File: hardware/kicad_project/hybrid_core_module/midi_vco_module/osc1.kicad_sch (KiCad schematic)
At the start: 57 parts, among them Q12 SSM2212, Q14 BF545A, Q15 2N7002, Q16 2N7002, U11 TL074, U12 LM311DR, U13 TL072

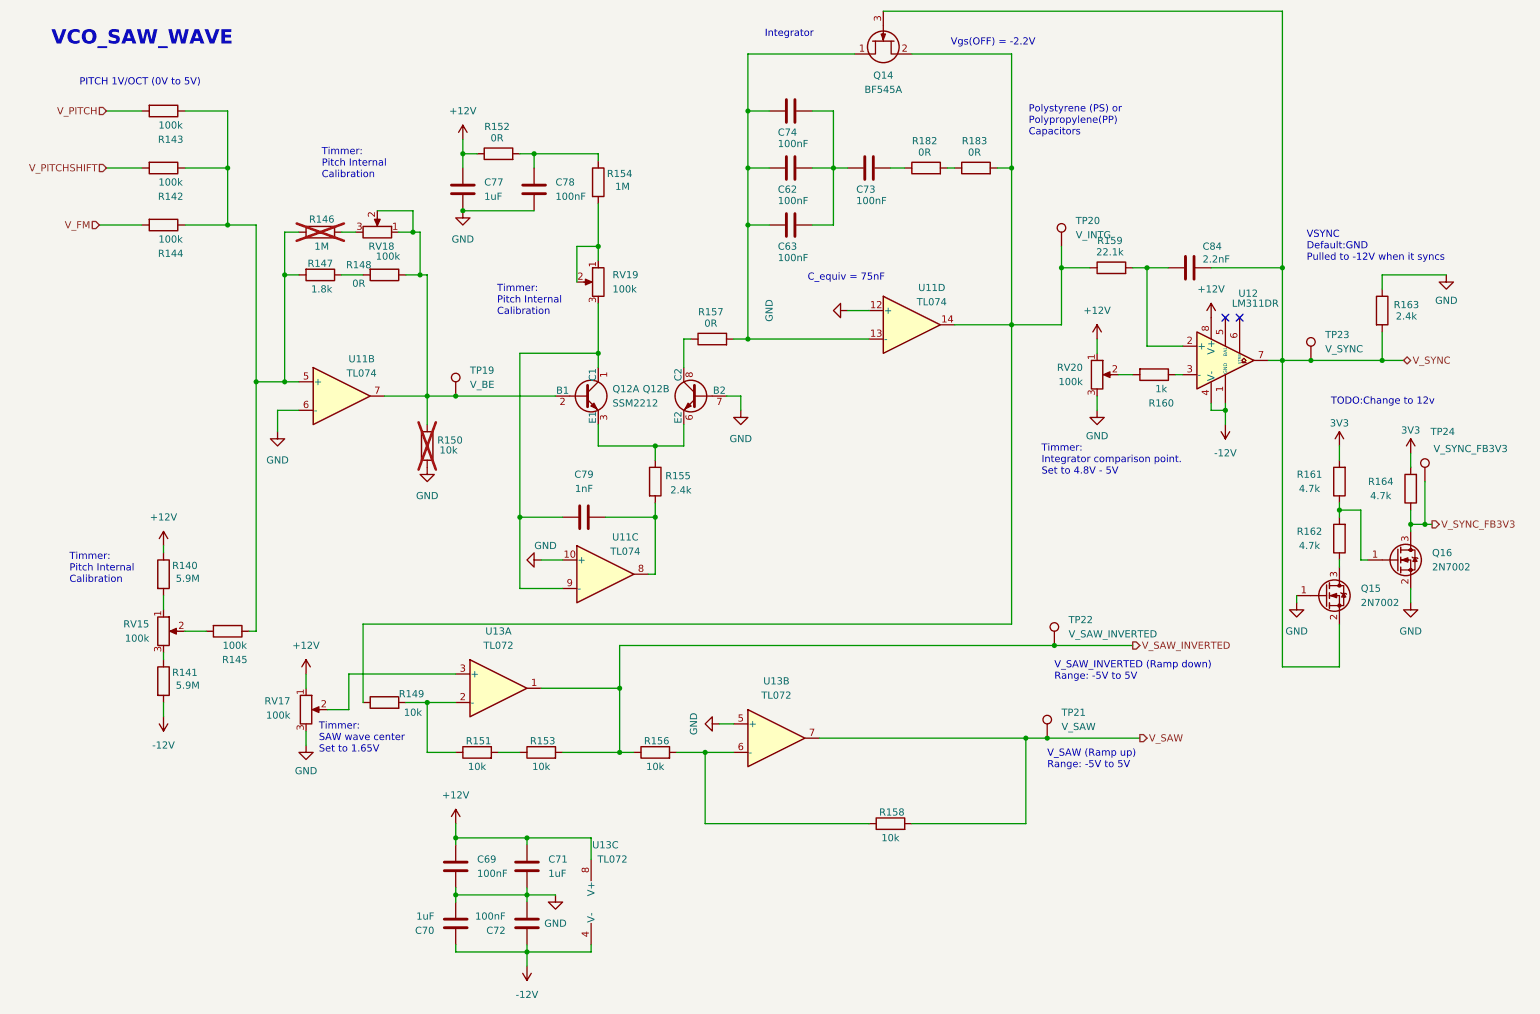
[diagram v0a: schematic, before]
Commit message: - placement done - routing 60%
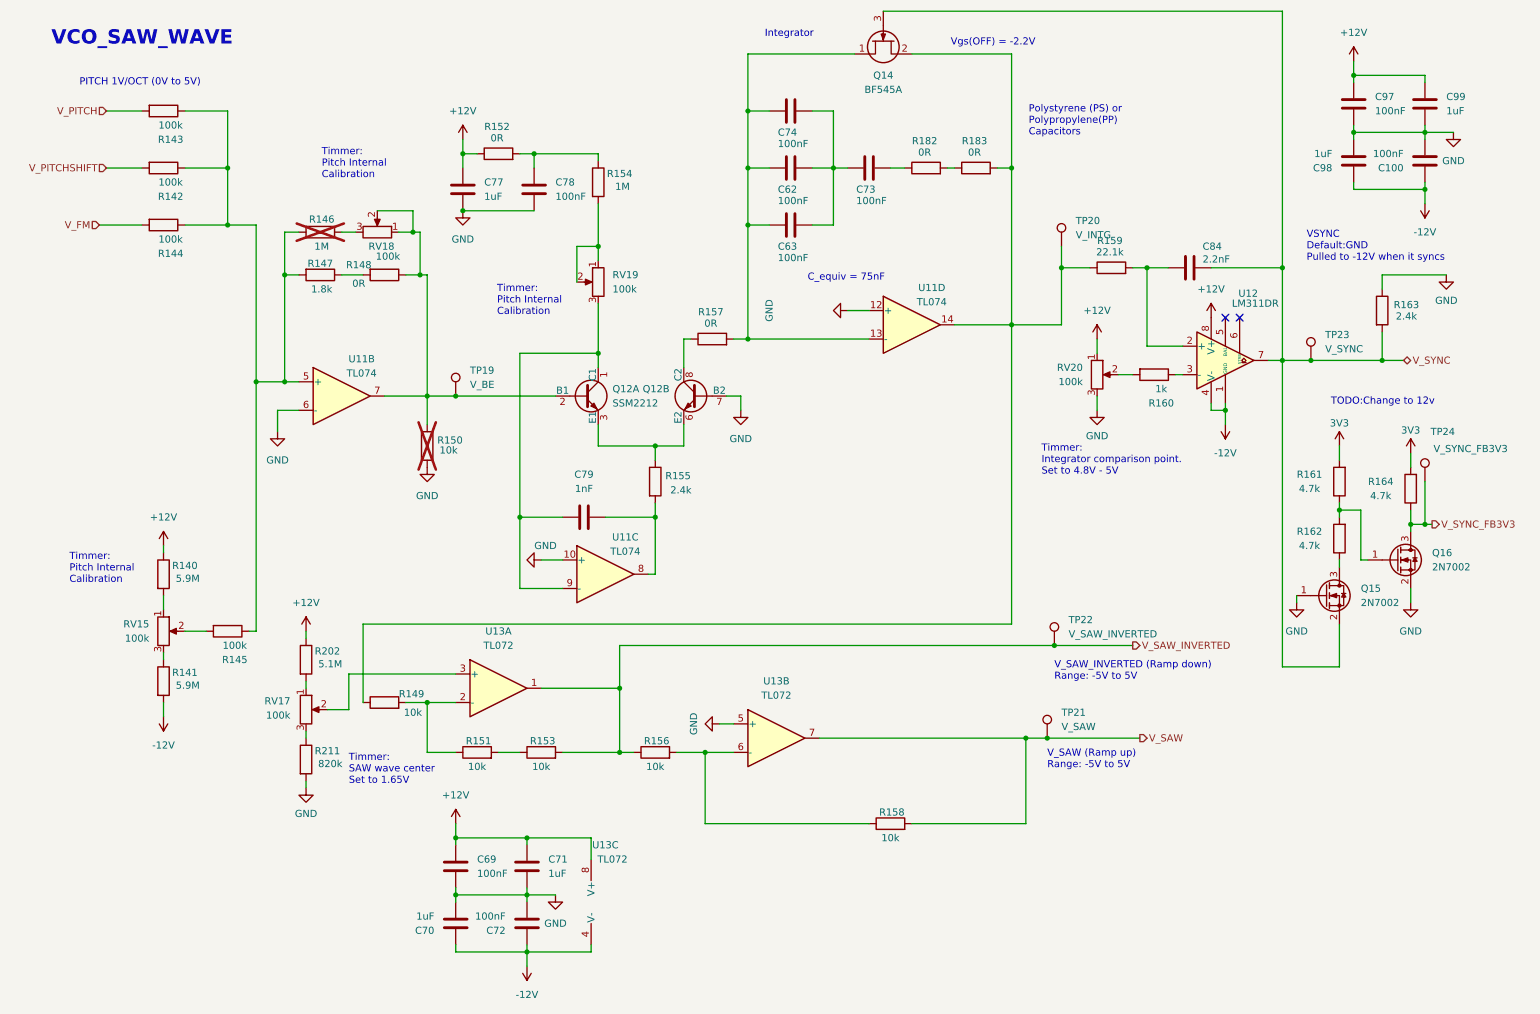
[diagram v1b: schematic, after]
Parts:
- added C100, C97: 100nF, Capacitor_SMD:C_0402_1005Metric, symbol Device:C
- added C98, C99: 1uF, Capacitor_SMD:C_0805_2012Metric, symbol Device:C
- added R202: 5.1M, Resistor_SMD:R_0402_1005Metric, symbol Device:R
- added R211: 820k, Resistor_SMD:R_0402_1005Metric, symbol Device:R
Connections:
- net +12V: now also C97.1, C99.1, R202.1; no longer RV17.1
- net -12V: now also C100.1, C98.1
- net GND: now also C100.2, C97.2, C98.2, C99.2, R211.2; no longer RV17.3
- new net: R202.2, RV17.1
- new net: R211.1, RV17.3

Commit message: routing continued.
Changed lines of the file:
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@@
 		(lib_id "power:+15V")
 		(at 41.91 111.76 0)
+		(mirror y)
 		(unit 1)
 		(exclude_from_sim no)
@@
 		(on_board yes)
 		(dnp no)
-		(fields_autoplaced yes)
 		(property "Reference" "#PWR0279"
 			(at 41.91 115.57 0)
